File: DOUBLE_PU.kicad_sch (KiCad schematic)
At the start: 7 parts, among them Q12 AO3400A, Q13 AO3401A, Q14 AO3401A

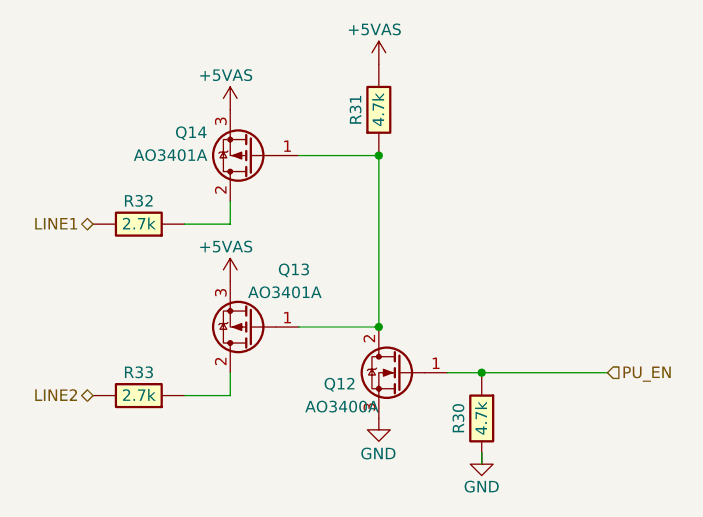
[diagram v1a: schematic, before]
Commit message: Export
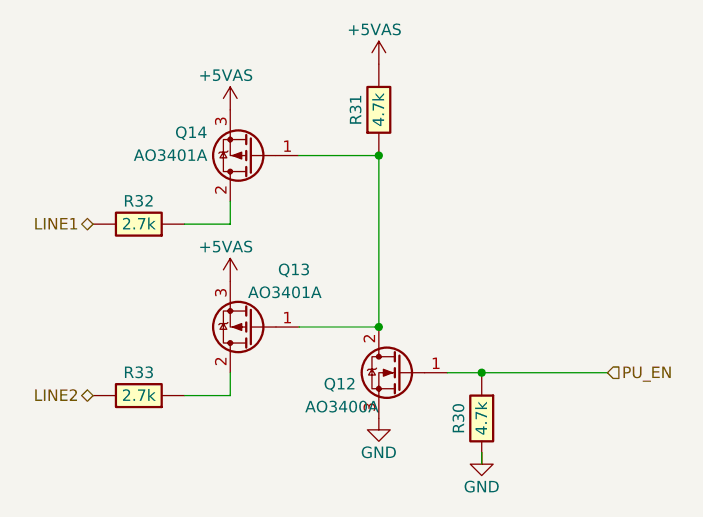
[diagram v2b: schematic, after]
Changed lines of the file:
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@@
       (effects (font (size 1.27 1.27)) hide)
     )
-    (property "Value" "GND" (at 153.6192 113.1634 0)
+    (property "Value" "GND" (at 153.67 113.03 0)
       (effects (font (size 1.27 1.27)))
     )
@@
         )
         (path "/63d2dd9f-d5ff-4811-a88d-0ba932475460/7c8c7251-8197-4c76-ae15-438276240430"
-          (reference "#PWR0160") (unit 1)
+          (reference "#PWR0211") (unit 1)
         )
       )
@@
         )
         (path "/63d2dd9f-d5ff-4811-a88d-0ba932475460/7c8c7251-8197-4c76-ae15-438276240430"
-          (reference "#PWR0161") (unit 1)
-        )
-      )
+          (reference "#PWR0212") (unit 1)
+        )
+      )
